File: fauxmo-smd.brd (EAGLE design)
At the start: 45.7 x 55.9 mm, 23 parts, among them J1 POWERJACKPTH, Q1 IRLB8721PBF, Q2 IRLB8721PBF, Q3 IRLB8721PBF, Q4 IRLB8721PBF

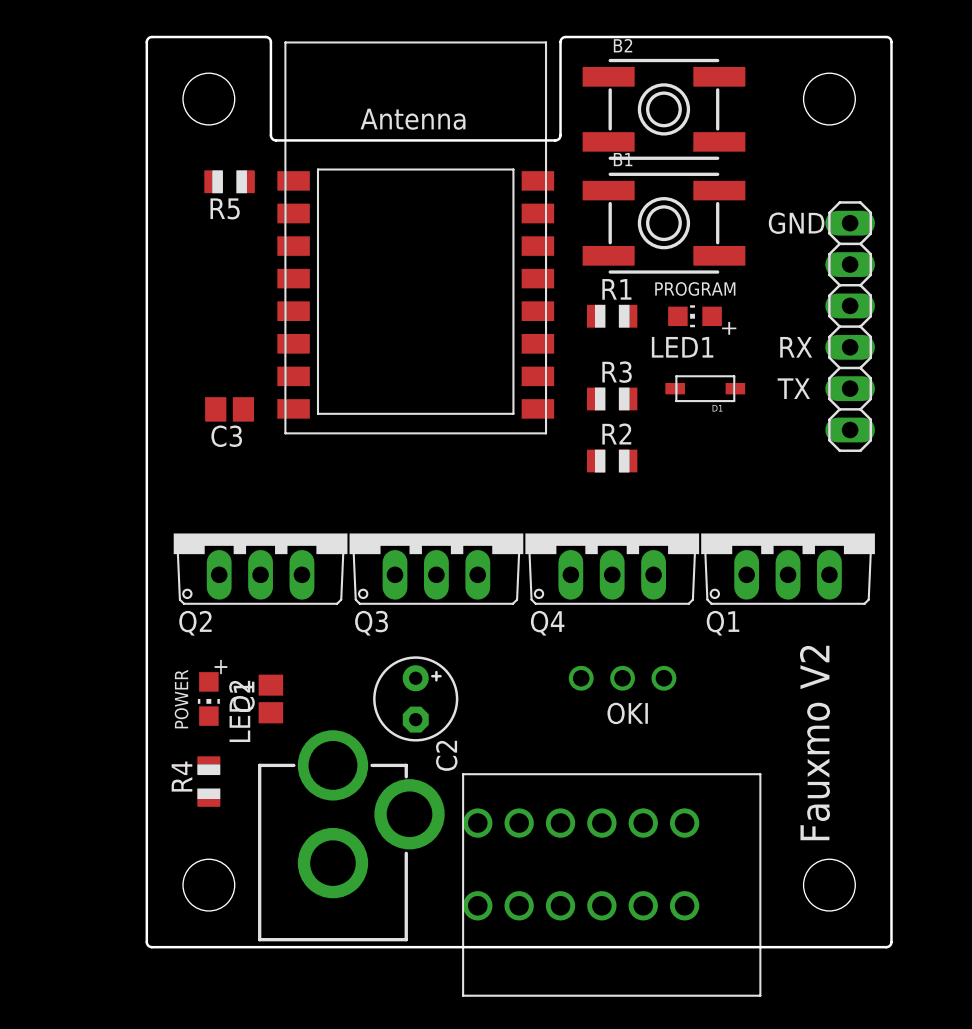
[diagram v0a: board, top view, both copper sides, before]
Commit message: Add files via upload
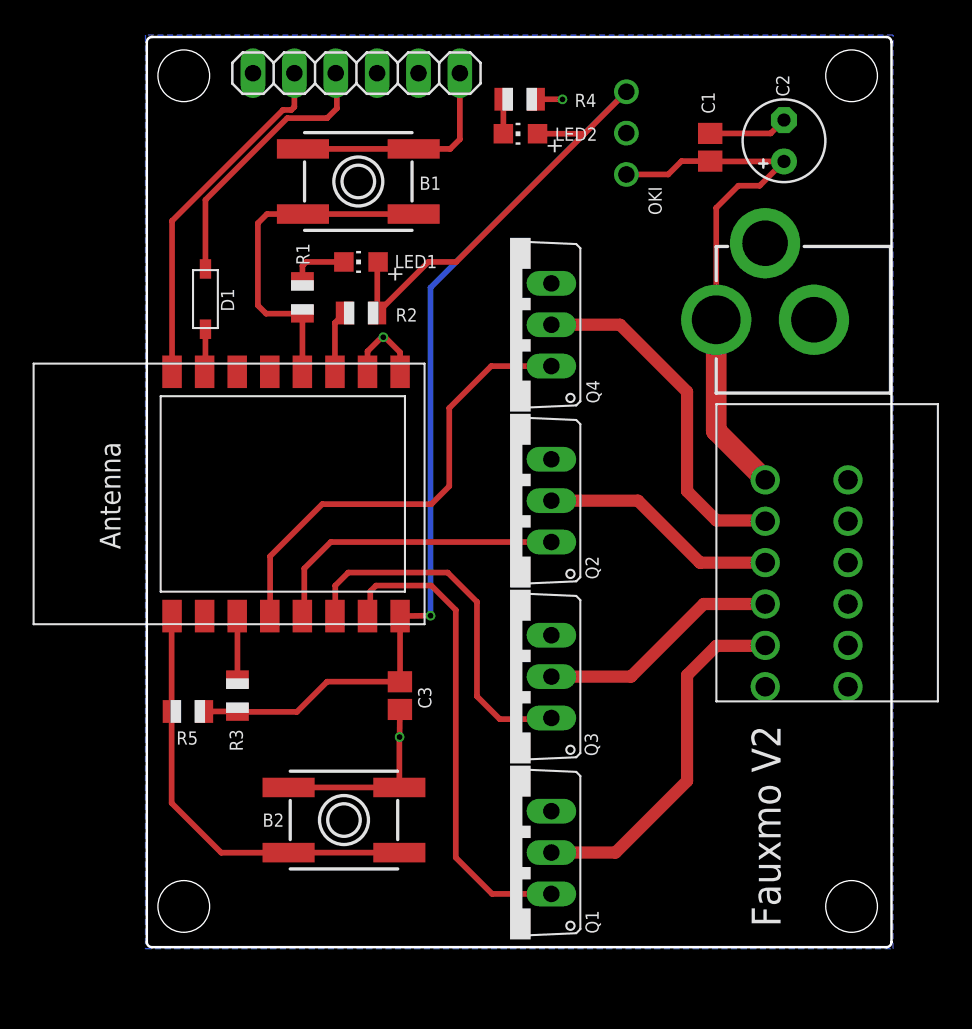
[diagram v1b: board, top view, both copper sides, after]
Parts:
- moved J1 55.4 mm to (47.4, 38.5), turned to 90 degrees
- moved B2 47.8 mm to (10.8, 7.80), turned to 180 degrees
- moved R4 46.0 mm to (21.6, 52.1), turned to 180 degrees
- moved C1 43.3 mm to (33.3, 49.1)
- moved C2 41.1 mm to (37.8, 49.5), turned to 90 degrees
- moved LED2 39.6 mm to (21.7, 49.9), turned to 90 degrees
- moved JP1 34.1 mm to (11.6, 53.7), turned to 180 degrees
- moved OKI 33.5 mm to (28.2, 50.0), turned to 270 degrees
- moved R5 32.6 mm to (1.25, 14.5), turned to 0 degrees
- moved D1 31.2 mm to (2.33, 39.8), turned to 270 degrees
- moved R3 29.3 mm to (4.29, 15.4), turned to 90 degrees
- moved Q1 26.0 mm to (21.0, 5.81), turned to 90 degrees
- moved U$2 24.8 mm to (29.2, 22.1)
- moved LED1 20.8 mm to (11.9, 42.1)
- moved C3 20.5 mm to (14.3, 15.4), turned to 270 degrees
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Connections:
- net BLUE: now also X1.6; no longer X1.5
- net GREEN: now also X1.5; no longer X1.7
- net RED: now also X1.4; no longer X1.6
- net WHITE: now also X1.7; no longer X1.4
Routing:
- net 3V3: track 0.00 -> 82.9 mm, vias 0 -> 1
- net GND: track 0.00 -> 37.2 mm, vias 0 -> 3
- net 12VDC: track 0.00 -> 33.3 mm
- net WHITE: track 0.00 -> 30.4 mm
- net RED: track 0.00 -> 30.2 mm
- net RESET: track 0.00 -> 26.7 mm
- net BLUE: track 0.00 -> 24.2 mm
- net WHITELED: track 0.00 -> 22.2 mm
- net TXD: track 0.00 -> 21.7 mm
- net REDLED: track 0.00 -> 21.7 mm
- net GPIO0: track 0.00 -> 21.4 mm
- net GREEN: track 0.00 -> 18.8 mm
- net RXDD: track 0.00 -> 16.8 mm
- net BLUELED: track 0.00 -> 15.0 mm
- net GREENLED: track 0.00 -> 14.7 mm
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- added copper zone on layer 16, net GND
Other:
- outline, holes or cut-outs redrawn
- board text added: "+12VDC"
- board text added: "BLUE"
- board text added: "GREEN"
- board text added: "POWER IN 12VDC 60W MAX"
- board text added: "PROGRAMING HEADER"
- board text added: "RED"
- board text added: "WHITE"
- board text removed: "POWER"
- board text removed: "PROGRAM"
